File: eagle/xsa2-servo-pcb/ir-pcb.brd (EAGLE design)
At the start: 96 x 85 mm, 62 parts, among them IC1 ATMEGA328P-AU, IC10 SK6812_SIDE, IC11 SK6812_SIDE, IC12 SK6812_SIDE, IC13 SK6812_SIDE, IC14 SK6812_SIDE, IC15 SK6812_SIDE, IC16 SK6812_SIDE, IC17 SK6812_SIDE, IC18 SK6812_SIDE, IC19 SK6812_SIDE, IC2 PL-IRM0101, IC3 PL-IRM0101, IC4 PL-IRM0101, IC5 PL-IRM0101, IC6 PL-IRM0101, IC7 PL-IRM0101, IC8 SK6812_SIDE, IC9 SK6812_SIDE, Q1 IRLML6402, Q2 IRFML8244, Q3 IRFML8244, Q4 IRFML8244, Q5 8MHz, Q6 IRFML8244

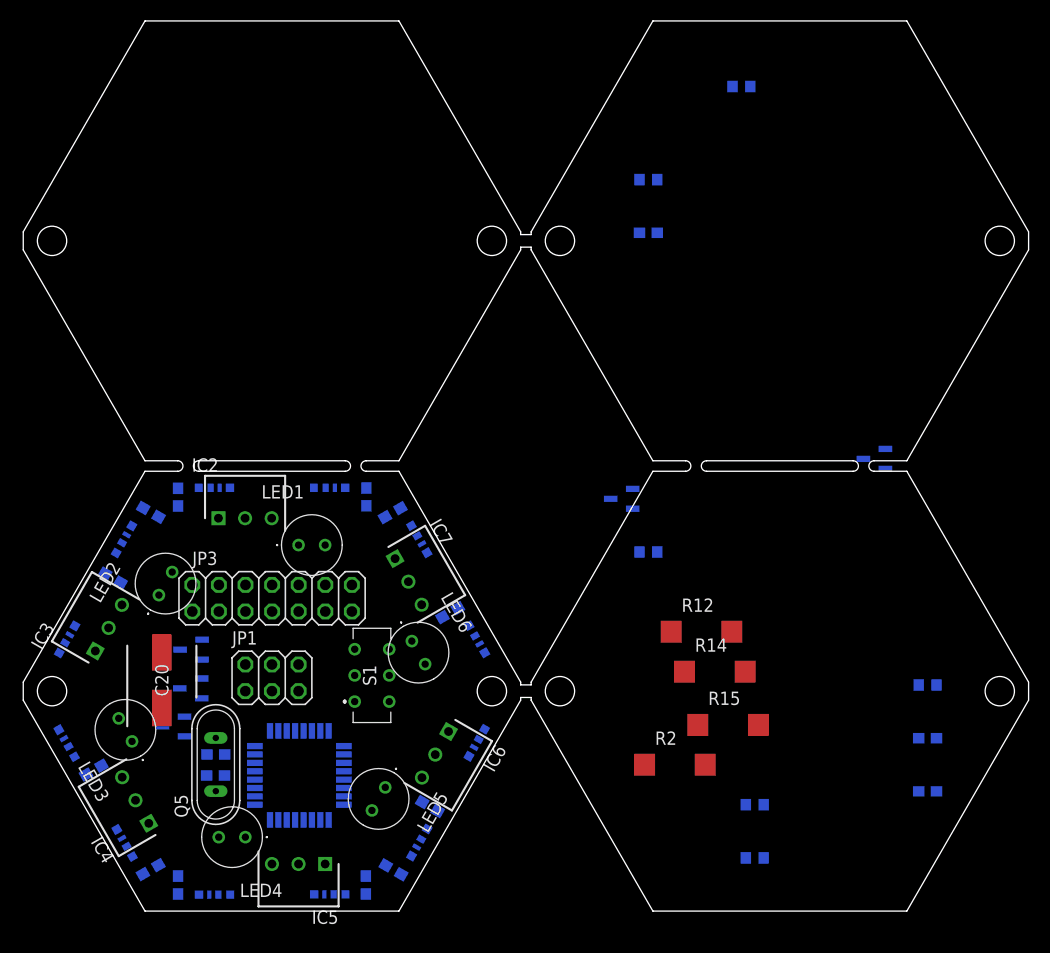
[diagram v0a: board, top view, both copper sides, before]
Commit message: [eagle] サーボ基板完成
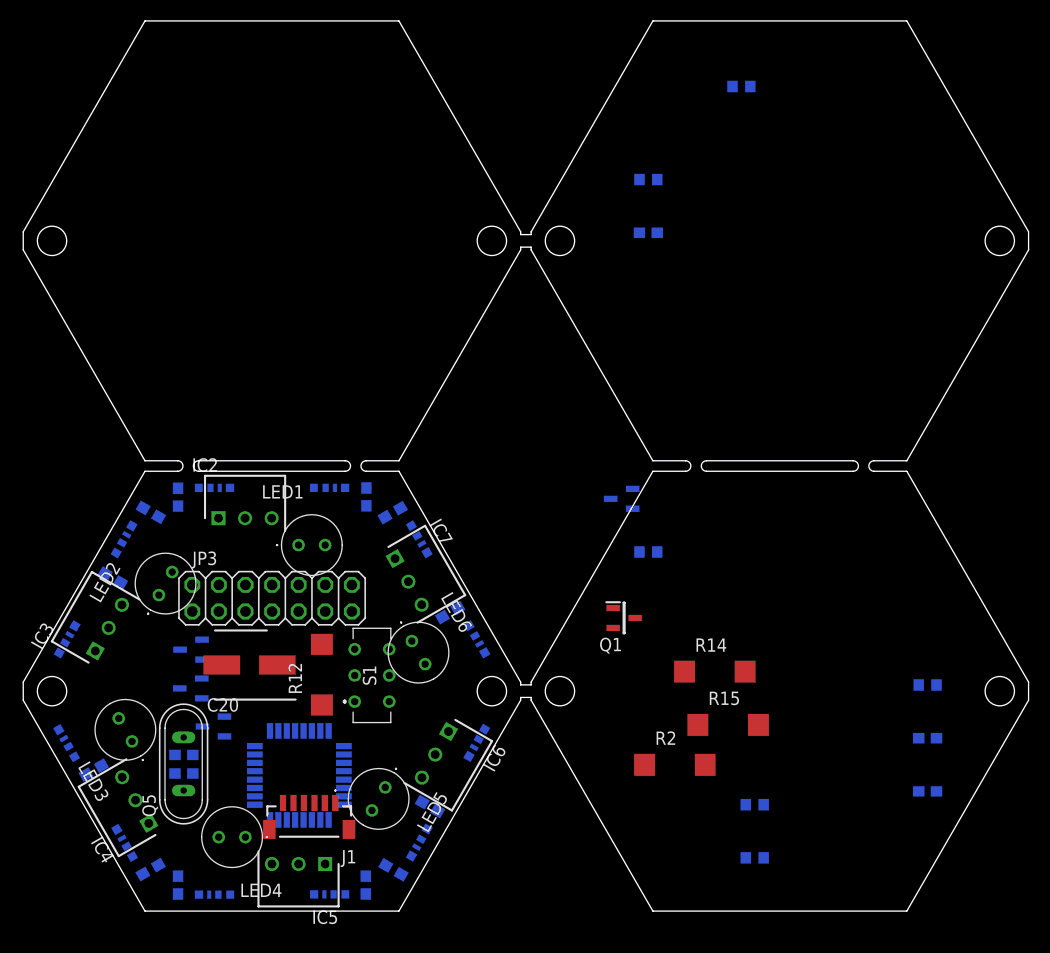
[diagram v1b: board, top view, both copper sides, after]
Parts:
- removed JP1: AVR ISP, pinhead:2X03
- added J1: BM06B-SRSS-TBT_LF__SN_, SamacSys_Parts:BM06BSRSSTBTLFSN
- moved R12 36.5 mm to (28.5, 22.6), turned to 90 degrees
- moved Q1 28.3 mm to (57.4, 28.0), flipped to the top
- moved C20 8.51 mm to (21.6, 23.5), turned to 180 degrees
- moved Q4 3.81 mm to (18.2, 17.6)
- moved Q5 3.07 mm to (15.3, 14.0)
- moved C4 3.05 mm to (15.3, 14.9)
- moved C3 3.03 mm to (15.3, 13.1)
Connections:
- net +3V3: now also J1.2; no longer JP1.2
- net GND: now also J1.6; no longer JP1.6
- net N$1: now also J1.1; no longer JP1.1
- net N$25: now also J1.5; no longer JP1.5
- net N$41: now also J1.4; no longer JP1.4
- net N$5: now also J1.3; no longer JP1.3
